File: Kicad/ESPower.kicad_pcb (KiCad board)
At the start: 2 copper layers, 82.4 x 15.2 mm, 36 parts, among them Q1 DMP2035U-7, Q2 FS8205A, U1 TP4056, U2 DW01A, U3 SPX3819M5-L-3-3, U4 TPS3839DBZ

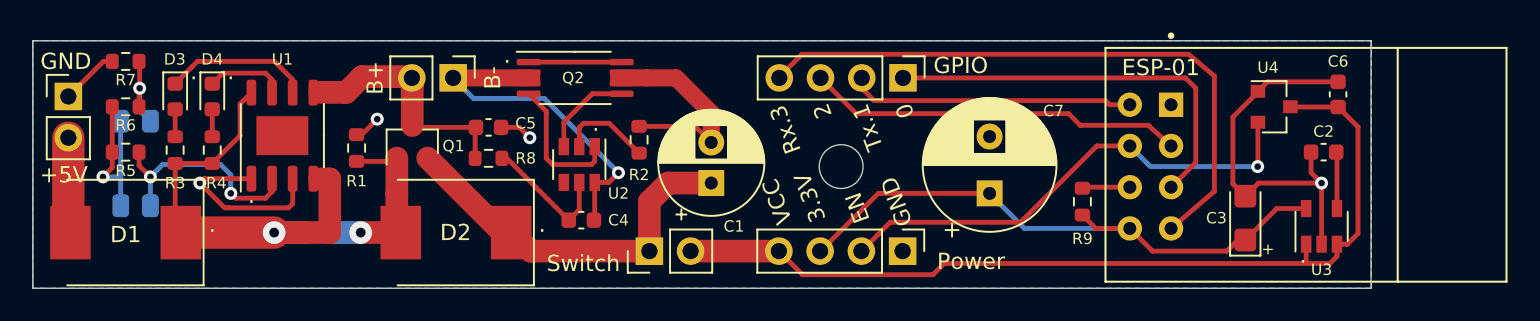
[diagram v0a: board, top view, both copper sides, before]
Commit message: Version 1.0
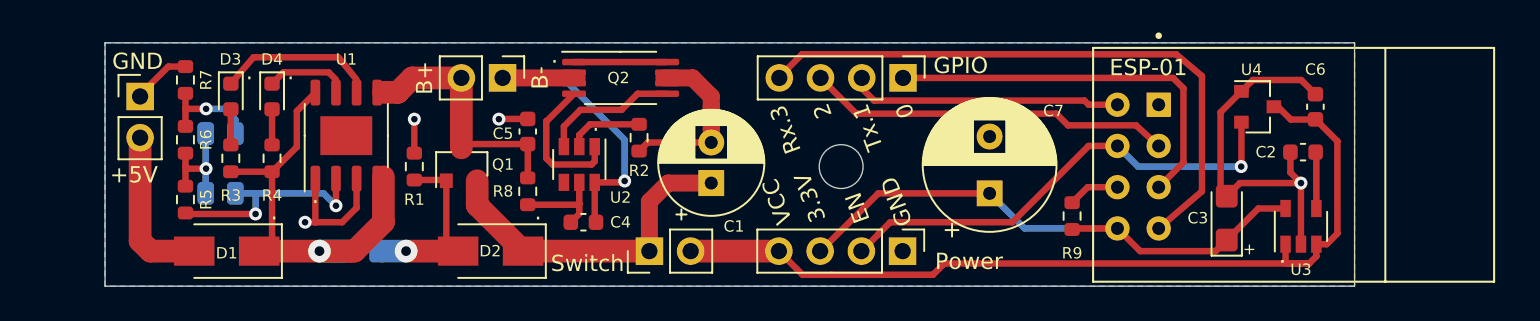
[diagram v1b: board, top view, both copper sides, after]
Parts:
- D1, D2: value SS34C -> SS34; footprint Diode_SMD:D_SMC -> Diode_SMD:D_SMA
- moved D1 6.33 mm to (89.4, 106.8)
- moved A 5.29 mm to (89.0, 103.3)
- moved B 5.29 mm to (89.0, 99.6)
- moved R5 4.70 mm to (86.9, 103.6), turned to 90 degrees
- moved GND 4.42 mm to (84.1, 97.3)
- moved R6 4.21 mm to (86.9, 99.9), turned to 90 degrees
- moved U1 3.94 mm to (96.8, 99.7)
- moved R7 3.86 mm to (86.9, 96.3), turned to 90 degrees
- moved R1 3.74 mm to (101.0, 101.6)
- moved R4 3.72 mm to (92.2, 101.1)
- moved D4 3.68 mm to (92.2, 97.3)
- moved R3 3.47 mm to (89.7, 101.1)
- moved D3 3.43 mm to (89.7, 97.3)
- moved Q1 3.35 mm to (103.9, 101.5)
- moved R8 3.15 mm to (108.0, 103.1), turned to 270 degrees
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- gave numbers to parts that had none: 1
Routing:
- net GND: track 55.9 -> 50.7 mm
- net Net-(D1-PadA): track 6.01 -> 9.95 mm
- net Net-(R5-Pad2): track 10.9 -> 7.04 mm
- net Net-(C4-Pad1): track 8.62 -> 5.87 mm
- net Net-(C1-Pad1): track 23.4 -> 20.6 mm
- net Net-(Q2-Pad5): track 5.79 -> 8.43 mm
- net Net-(C4-Pad2): track 22.3 -> 20.6 mm
- net +3V3: track 37.3 -> 36.0 mm
- net Net-(J3-Pad2): track 30.5 -> 29.3 mm
- net Net-(R6-Pad2): track 5.13 -> 6.24 mm
- net Net-(R2-Pad1): track 5.74 -> 4.67 mm
- net VDD: track 55.7 -> 54.7 mm
- net Net-(D3-Pad1): track 9.44 -> 10.3 mm
- net Net-(J5-Pad4): track 38.6 -> 37.8 mm
- net Net-(J5-Pad3): track 23.3 -> 22.5 mm
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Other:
- board size 82.4 x 15.2 mm -> 77 x 15 mm
- net class Default: trace_width 0.3 -> 0.4
- board text added: "On: VCC=Input|Batt Off: VCC=Batt"
- board text removed: "0: VCC=Batt 1: VCC=Input|Batt"
